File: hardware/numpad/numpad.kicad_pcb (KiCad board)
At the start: 2 copper layers, 83 x 124 mm, 116 parts, among them J1 USB_C_Receptacle_USB2.0_16P, J2 Conn_01x03, J3 Conn_01x04, Q1 BSS138, Q2 BSS138, SW1 BOOTSEL, SW2 RESET, SW3 RotaryEncoder_Switch, U1 NCP1117-3.3_SOT223, U2 USBLC6-2SC6, U3 RP2040, U4 W25Q128JVS, U5 74AHCT1G125, Y1 12MHz

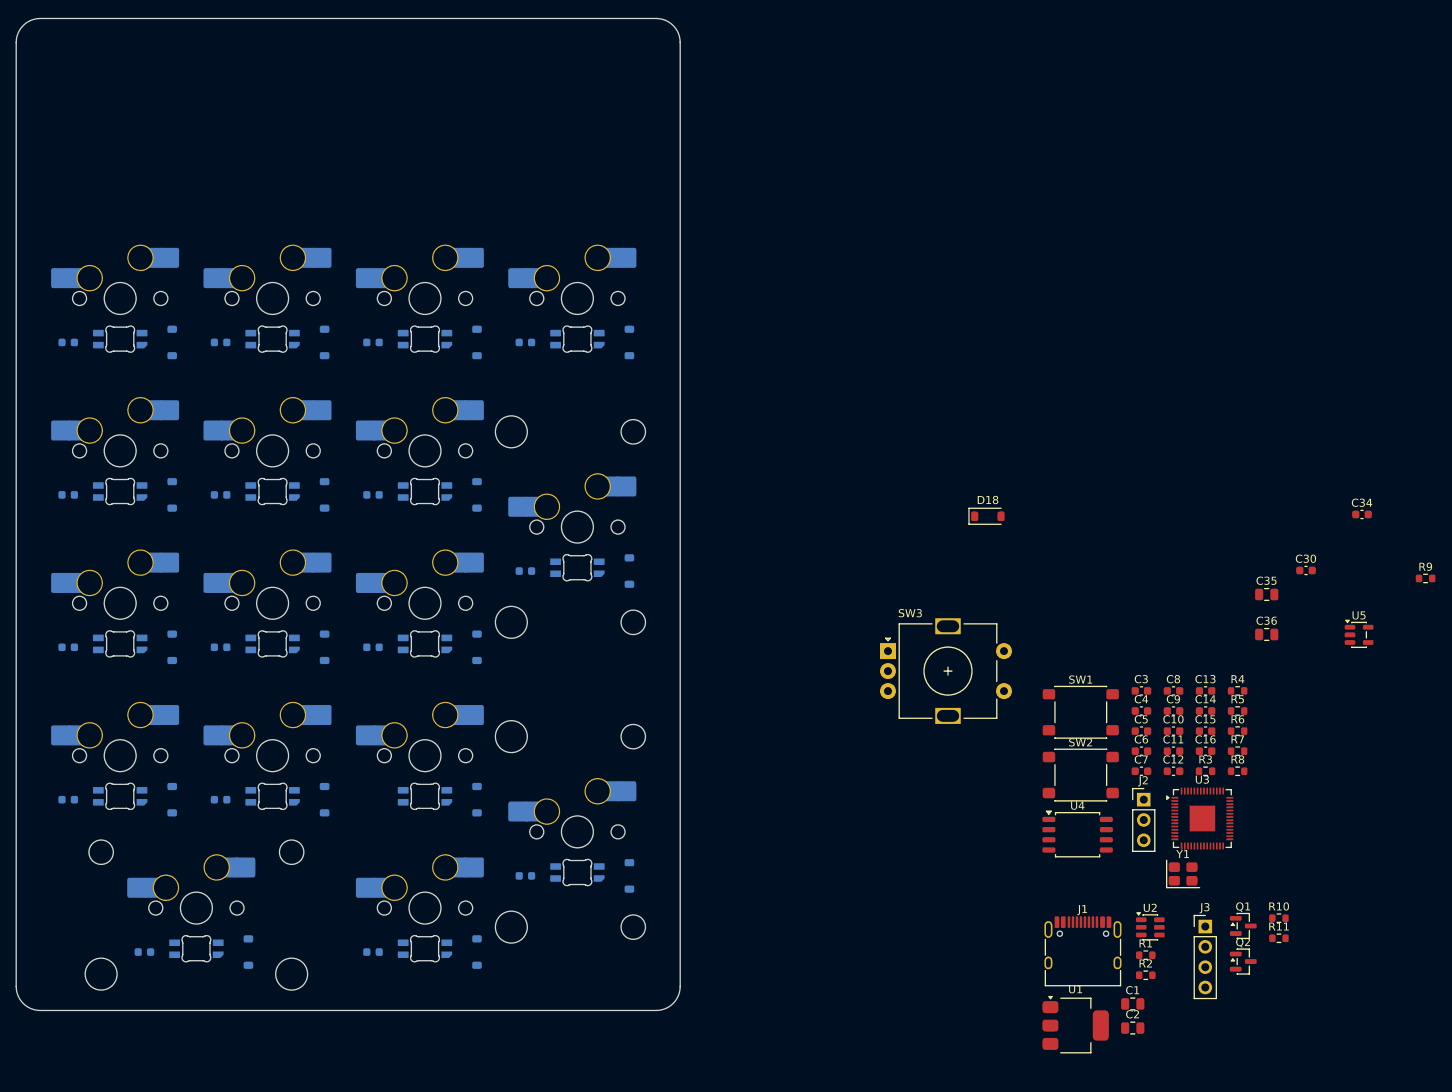
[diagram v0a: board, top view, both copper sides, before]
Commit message: USB entry and MCU cluster
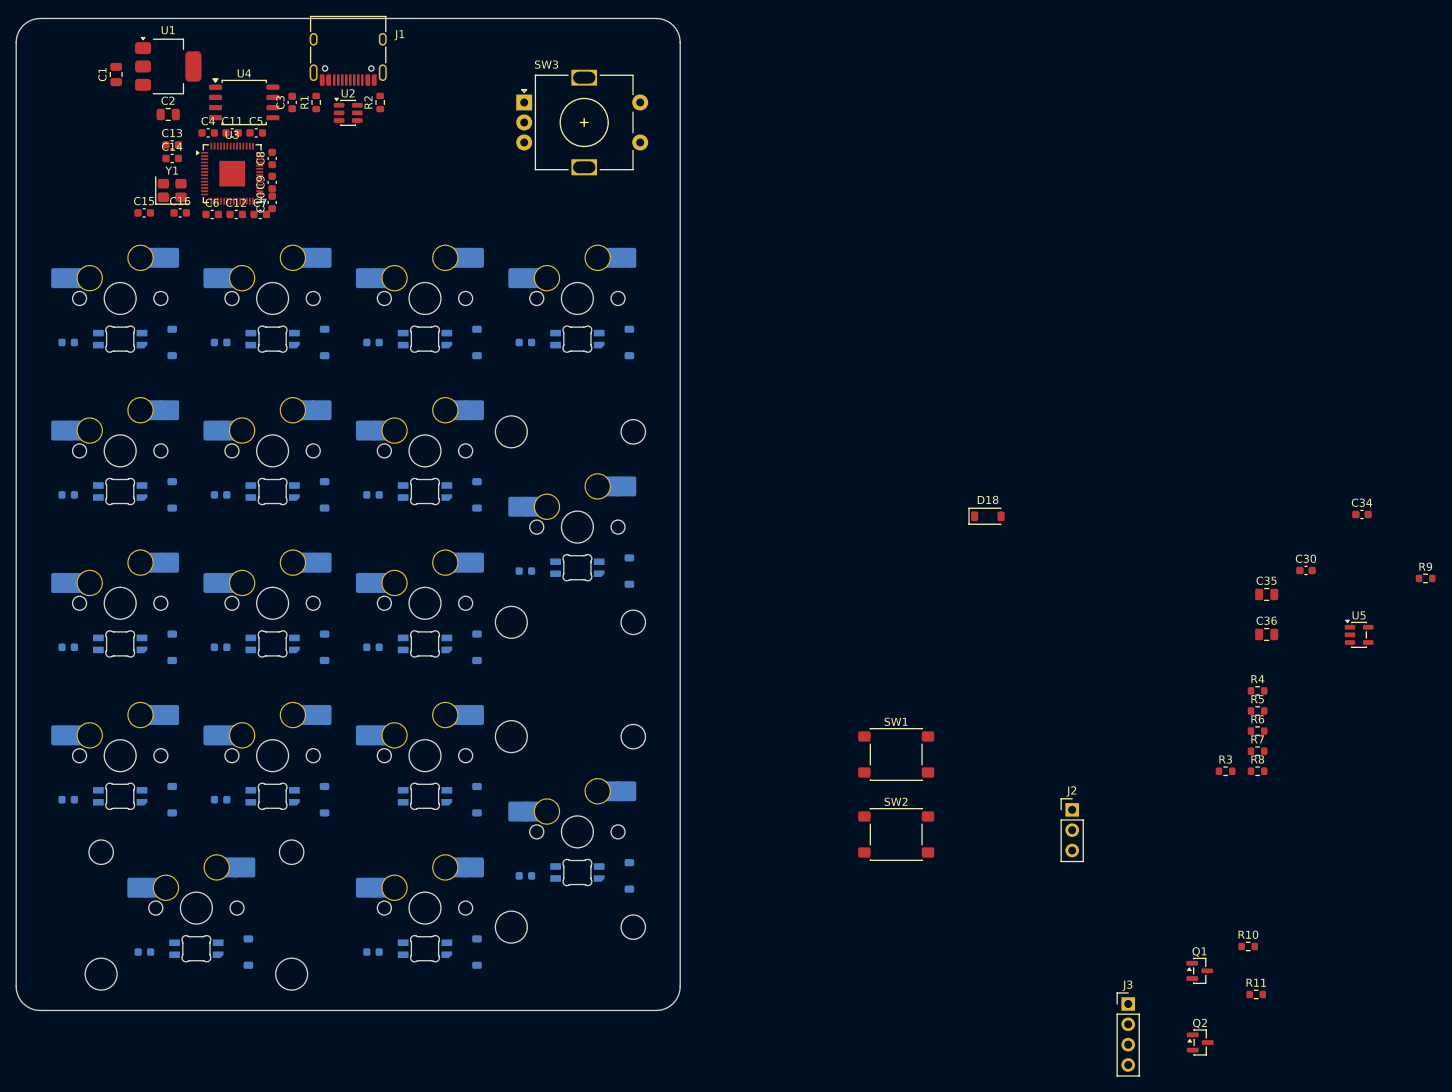
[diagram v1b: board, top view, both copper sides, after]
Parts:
- C11, C3: value 1u -> 100n
- moved C1 172.2 mm to (59.5, 12.0), turned to 90 degrees
- moved C2 166.1 mm to (66.0, 17.0)
- moved U1 165.0 mm to (66.0, 11.0)
- moved Y1 152.5 mm to (66.5, 26.5)
- moved R1 148.7 mm to (84.5, 15.5), turned to 90 degrees
- moved C15 147.6 mm to (63.0, 29.3)
- moved C14 146.5 mm to (66.5, 22.5)
- moved C13 146.1 mm to (66.5, 20.8)
- moved J1 145.9 mm to (88.5, 8.65), turned to 180 degrees
- moved U3 145.6 mm to (74.0, 24.4)
- moved R2 145.1 mm to (92.5, 15.5), turned to 90 degrees
- moved C16 144.8 mm to (67.5, 29.3)
- moved U2 142.9 mm to (88.5, 16.8)
- moved C11 140.8 mm to (74.0, 19.3)
- moved U4 138.7 mm to (75.5, 15.5)
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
